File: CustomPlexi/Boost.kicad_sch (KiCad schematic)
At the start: 8 parts, among them U1 TL074

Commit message: Signal chain ok except separated volumes
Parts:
- C8, C9: footprint Capacitor_SMD:C_0603_1608Metric_Pad1.08x0.95mm_HandSolder -> Capacitor_SMD_AKL:C_0603_1608Metric
- R10, R11, R8, R9: footprint Resistor_SMD:R_0603_1608Metric_Pad0.98x0.95mm_HandSolder -> Resistor_SMD_AKL:R_0603_1608Metric
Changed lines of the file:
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@@
       (effects (font (size 1.27 1.27)))
     )
-    (property "Footprint" "Capacitor_SMD:C_0603_1608Metric_Pad1.08x0.95mm_HandSolder" (at 133.35 93.0148 0)
+    (property "Footprint" "Capacitor_SMD_AKL:C_0603_1608Metric" (at 133.35 93.0148 0)
       (effects (font (size 1.27 1.27)) hide)
     )
@@
       (effects (font (size 1.27 1.27)))
     )
-    (property "Footprint" "Resistor_SMD:R_0603_1608Metric_Pad0.98x0.95mm_HandSolder" (at 146.05 93.98 0)
+    (property "Footprint" "Resistor_SMD_AKL:R_0603_1608Metric" (at 146.05 93.98 0)
       (effects (font (size 1.27 1.27)) hide)
     )
@@
       (effects (font (size 1.27 1.27)) (justify right))
     )
-    (property "Footprint" "Resistor_SMD:R_0603_1608Metric_Pad0.98x0.95mm_HandSolder" (at 116.84 76.2 0)
+    (property "Footprint" "Resistor_SMD_AKL:R_0603_1608Metric" (at 116.84 76.2 0)
       (effects (font (size 1.27 1.27)) hide)
     )
@@
       (effects (font (size 1.27 1.27)))
     )
-    (property "Footprint" "Capacitor_SMD:C_0603_1608Metric_Pad1.08x0.95mm_HandSolder" (at 110.744 101.9048 0)
+    (property "Footprint" "Capacitor_SMD_AKL:C_0603_1608Metric" (at 110.744 101.9048 0)
       (effects (font (size 1.27 1.27)) hide)
     )
@@
       (effects (font (size 1.27 1.27)) (justify right))
     )
-    (property "Footprint" "Resistor_SMD:R_0603_1608Metric_Pad0.98x0.95mm_HandSolder" (at 167.894 88.9 0)
+    (property "Footprint" "Resistor_SMD_AKL:R_0603_1608Metric" (at 167.894 88.9 0)
       (effects (font (size 1.27 1.27)) hide)
     )
@@
       (effects (font (size 1.27 1.27)))
     )
-    (property "Footprint" "Resistor_SMD:R_0603_1608Metric_Pad0.98x0.95mm_HandSolder" (at 106.68 102.87 0)
-      (effects (font (size 1.27 1.27)) hide)
-    )
+    (property "Footprint" "Resistor_SMD_AKL:R_0603_1608Metric" (at 106.68 102.87 0)
+      (effects (font (size 1.27 1.27)) hide)
+    )

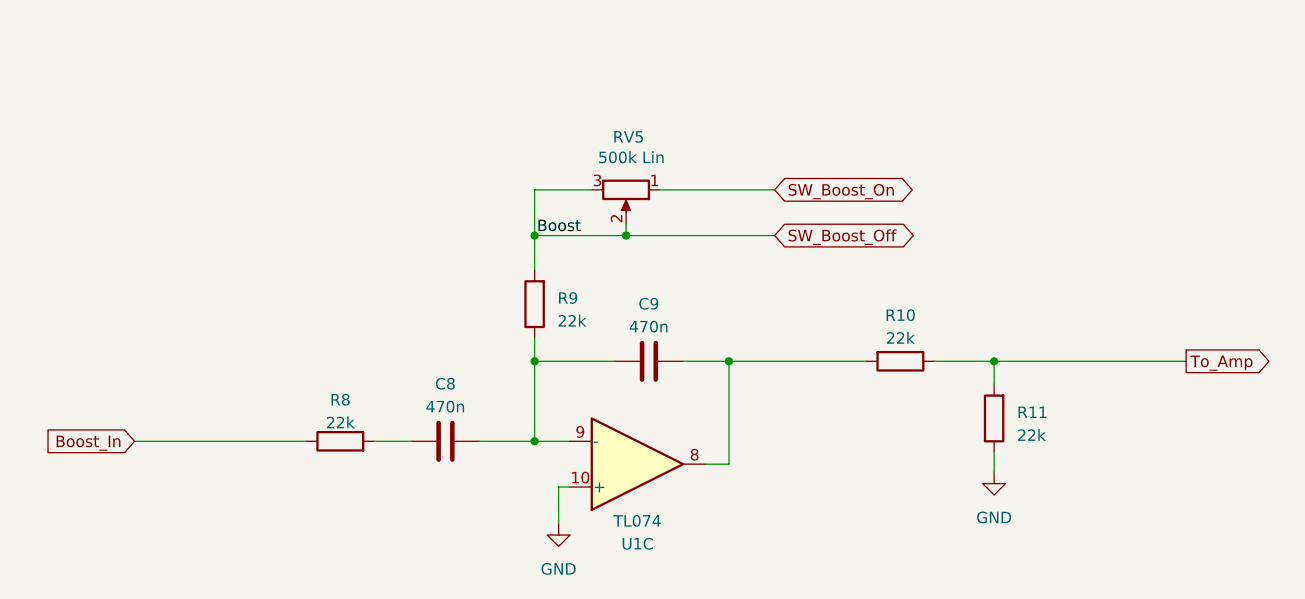
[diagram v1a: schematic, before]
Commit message: some changes
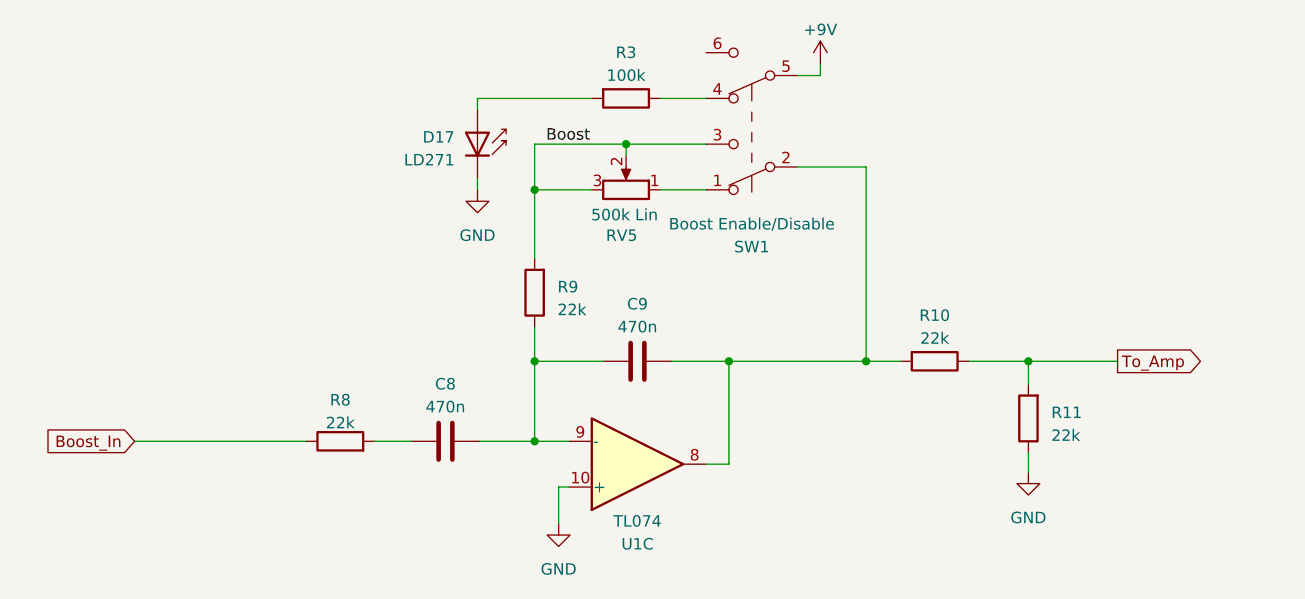
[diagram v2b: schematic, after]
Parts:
- added D17: LD271, LED_THT:LED_D5.0mm_IRGrey, symbol LED:LD271
- added R3: 100k, Resistor_SMD_AKL:R_0603_1608Metric, symbol PCM_Resistor_AKL:R_0603
- added SW1: Boost Enable/Disable, symbol Switch:SW_Push_DPDT
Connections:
- net GND: now also D17.1 (K)
- net at C9.2, R10.2, U1.8: now also SW1.2 (B)
- net SW_Boost_Off renamed Boost
- net Boost: now also SW1.3 (C)
- net SW_Boost_On: no longer names the net of RV5.1
- net SW_Boost_On: now also SW1.1 (A)
- new net: R3.1, SW1.4 (A)
- new net: D17.2 (A), R3.2
- new net +9V: SW1.5 (B)
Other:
- moved on the sheet: C9, R10, R11, R9, RV5
